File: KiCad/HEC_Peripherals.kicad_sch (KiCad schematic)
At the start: 19 parts, among them J2 Conn_02x12_Odd_Even, J6 DE9_Plug_MountingHoles, J7 AudioJack3, J8 NES_Port_Male, U43 74LS06, U44 74LS541, Y1 Crystal

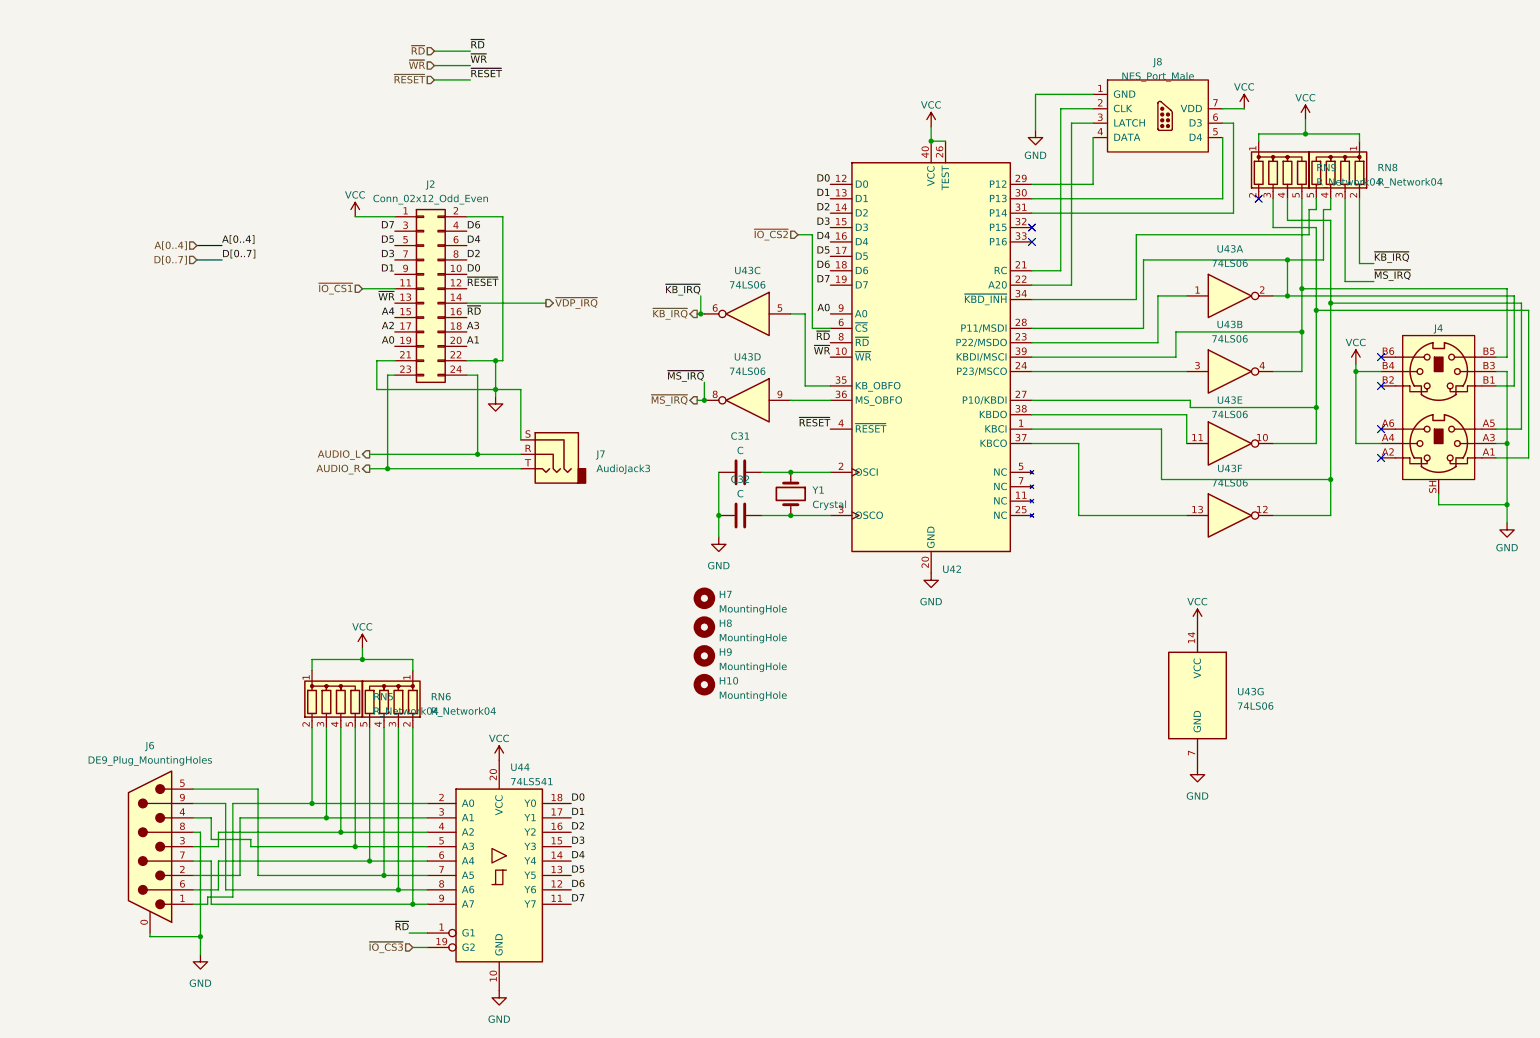
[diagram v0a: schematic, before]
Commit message: Updates to circuit
Updates to the second gen circuit
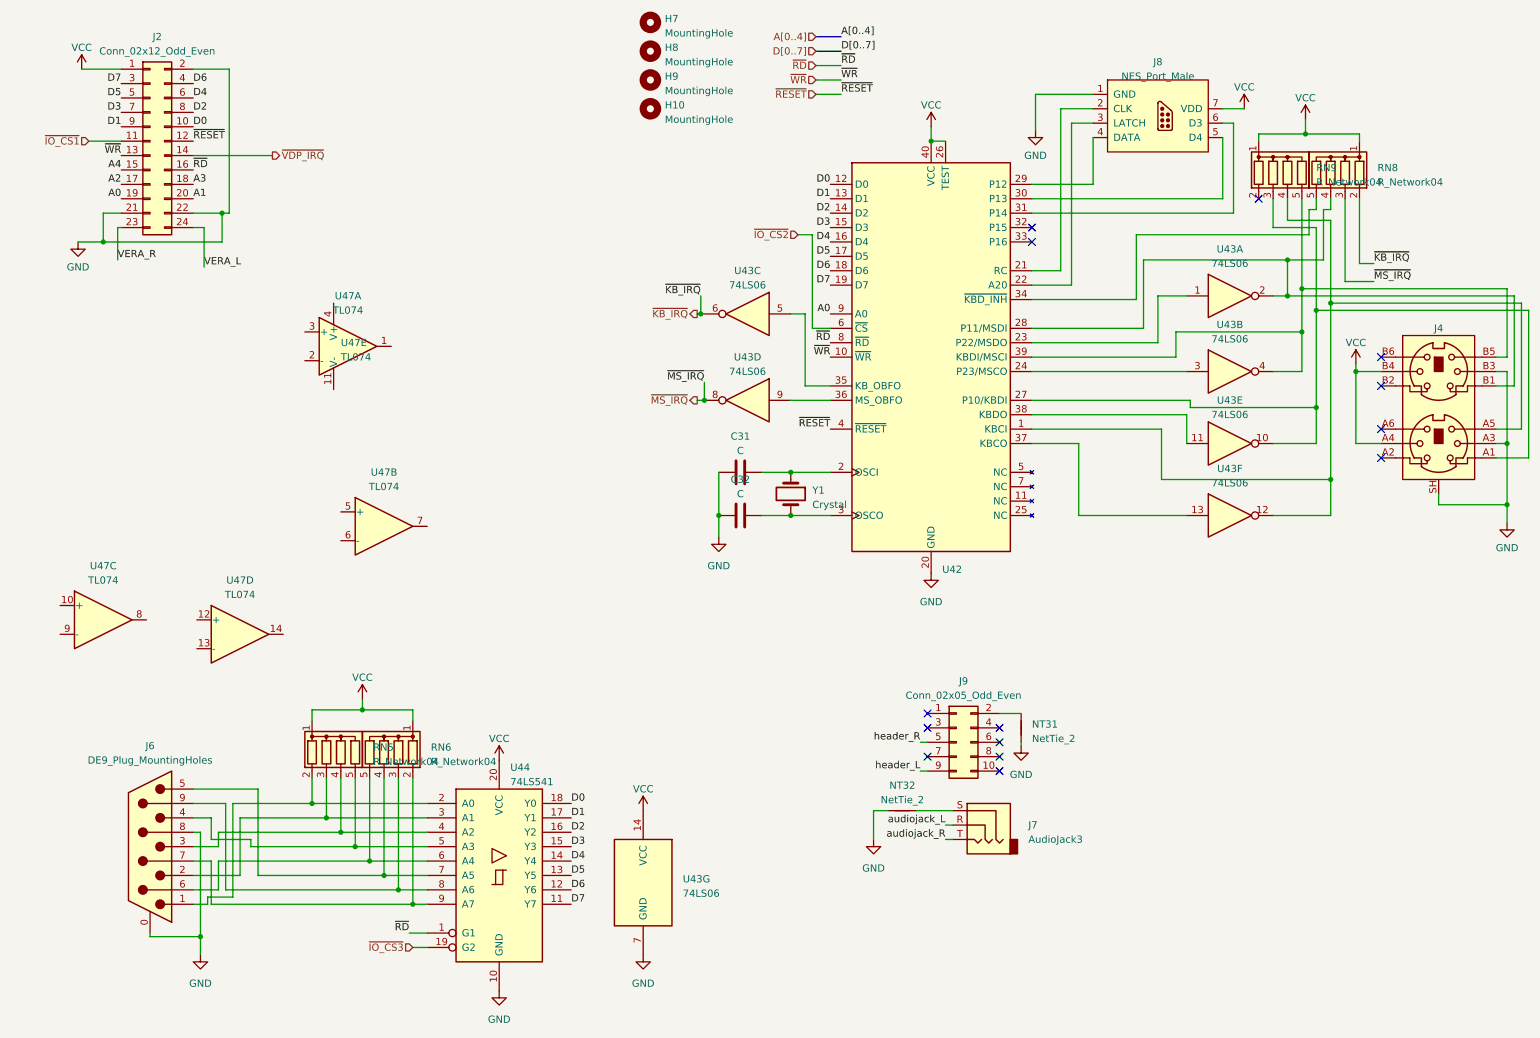
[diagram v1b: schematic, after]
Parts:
- added J9: Conn_02x05_Odd_Even, symbol Connector_Generic:Conn_02x05_Odd_Even
- added NT31, NT32: NetTie_2, symbol Device:NetTie_2
- added U47: TL074, symbol Amplifier_Operational:TL074
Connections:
- net GND: now also NT31.1, NT32.1; no longer J7.S
- net AUDIO_L renamed VERA_L
- net VERA_L: no longer J7.R
- net AUDIO_R renamed VERA_R
- net VERA_R: no longer J7.T
- new net: J7.S, NT32.2
- new net: J9.2 (Pin_2), NT31.2
- new net audiojack_L: J7.R
- new net audiojack_R: J7.T
- new net header_L: J9.9 (Pin_9)
- new net header_R: J9.5 (Pin_5)
- no-connect marks 7 -> 14
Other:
- moved on the sheet: H10, H7, H8, H9, J2, RN5, RN6, U43G
